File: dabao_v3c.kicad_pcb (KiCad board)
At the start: 6 copper layers, 17.8 x 21.1 mm, 69 parts, among them J1 USB_C_Receptacle_USB2.0_16P, Q1 LP0404N3T5G, Q2 LN237N3T5G, SW1 SKTAAAE010, SW2 SKTAAAE010, U1 baochip1x, U3 SMD IC PMIC;DCDC Buck-ADJ-1A,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, U4 XIAO-HALF-HOLE-23P, U5 SGM7222YWQ10/TR, U7 SGM40567-4.2XG/TR, U8 TPS22916CYFPR, U9 SMD IC PMIC;DCDC Buck-ADJ-1A,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, Y2 48.000MHz

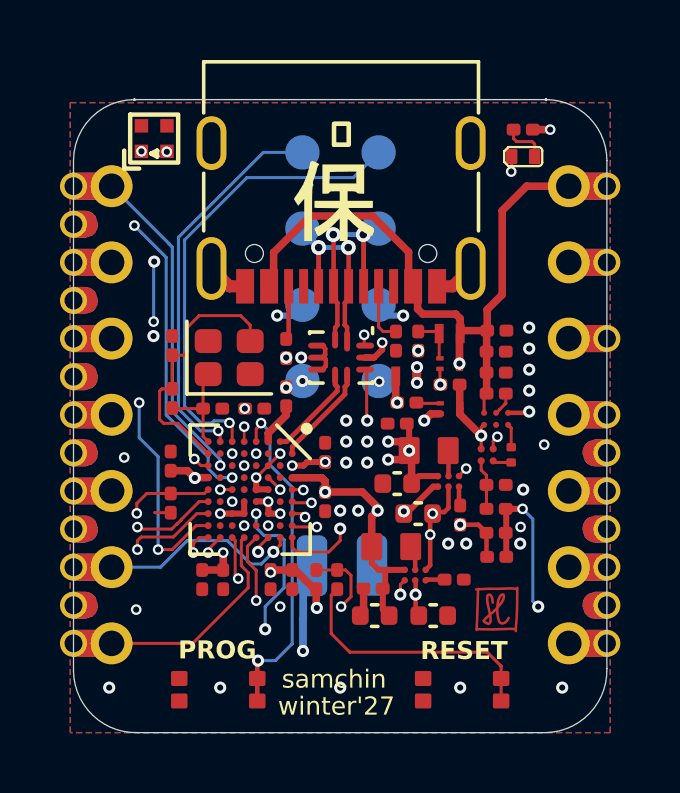
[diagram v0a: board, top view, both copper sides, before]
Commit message: nearly final
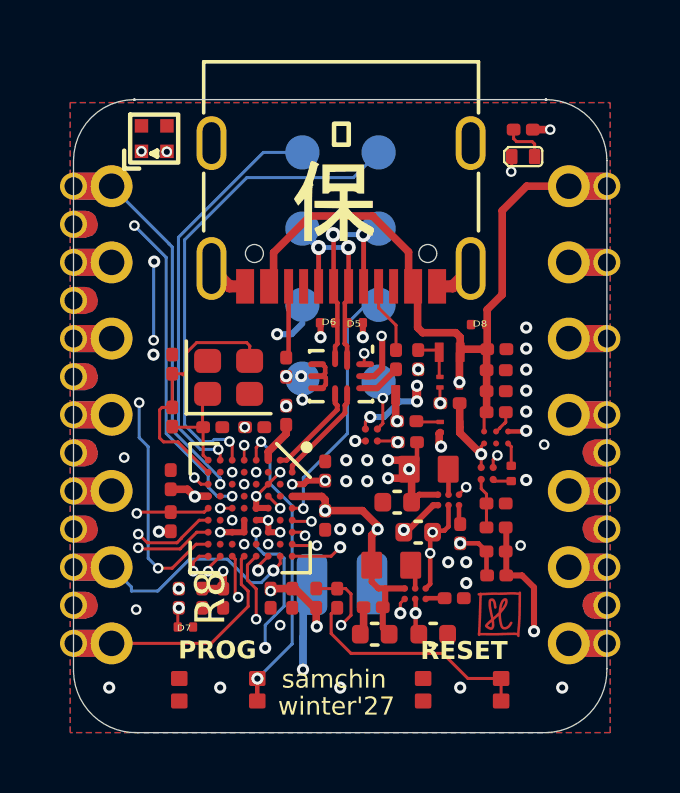
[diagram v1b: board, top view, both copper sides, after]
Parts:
- added D5: B74121U0055M060, xiao:ESD-0201, F.Cu at (132.5, 66.8)
- added D6: B74121U0055M060, xiao:ESD-0201, F.Cu at (131.6, 66.8)
- added D7: DF2B7ASL,L3F, xiao:ESD-0201, F.Cu at (126.8, 77.0)
- added D8: DF2B7ASL,L3F, xiao:ESD-0201, F.Cu at (136.6, 66.9)
- added R8: 5.1k, 1%, Resistor_SMD:R_0201_0603Metric, F.Cu at (126.6, 76.0)
- added U2: TPS22916CYFPR, xiao:WLCSP4-0.4-0.77X0.77X0.33MM, F.Cu at (133.0, 70.6)
- moved C20 0.71 mm to (134.2, 70.8)
- moved Y2 0.66 mm to (128.3, 68.7)
- moved C10 0.62 mm to (126.4, 68.2)
- moved C13 0.62 mm to (126.3, 73.5)
- moved C14 0.62 mm to (135.1, 77.2)
- moved C15 0.62 mm to (131.5, 73.4)
- moved C17 0.62 mm to (133.2, 77.2)
- moved C22 0.62 mm to (137.2, 68.4)
- moved C26 0.62 mm to (137.2, 75.3)
- moved C3 0.62 mm to (137.2, 69.1)
- moved C5 0.62 mm to (130.2, 69.9)
- moved C9 0.62 mm to (131.5, 71.8)
- moved L1 0.62 mm to (133.7, 74.9)
- moved L3 0.62 mm to (134.9, 71.7)
- moved R13 0.62 mm to (137.2, 73.7)
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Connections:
- net /PB3 renamed /PB3/WS2812_PWR_EN
- D1 pad 4: VSYS -> Net-(D1-VDD)
- U5 pad 10: /PC13 -> /PC13/BOOT
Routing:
- net Net-(D1-VDD): track 0.00 -> 20.6 mm, vias 0 -> 2
- net /PC13/BOOT: track 0.00 -> 20.5 mm, vias 0 -> 4
- net /PC13: track 16.9 -> 0.00 mm, vias 3 -> 0
- net VSYS: track 21.6 -> 7.20 mm
- net /PC5: track 9.90 -> 14.1 mm
- net /PA7/ADC3: track 19.8 -> 18.1 mm, vias 4 -> 3
- net VBUS: track 28.1 -> 29.7 mm
- net /PB3/WS2812_PWR_EN: track 7.21 -> 8.60 mm
- net /PB9: track 13.3 -> 12.0 mm
- net /RST_N: track 15.2 -> 13.9 mm
- net /PB5: track 9.04 -> 8.04 mm, vias 2 -> 1
- net /PC4: track 16.4 -> 17.4 mm
- net /PC1: track 18.4 -> 19.4 mm
- net /PC2: track 17.3 -> 18.3 mm
- net GND: track 15.6 -> 16.6 mm, vias 37 -> 40
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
